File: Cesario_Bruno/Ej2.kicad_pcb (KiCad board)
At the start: 2 copper layers, 38.7 x 31.4 mm, 4 parts, among them P1 CONN_01X14, P2 CONN_01X14, X1 XTAL

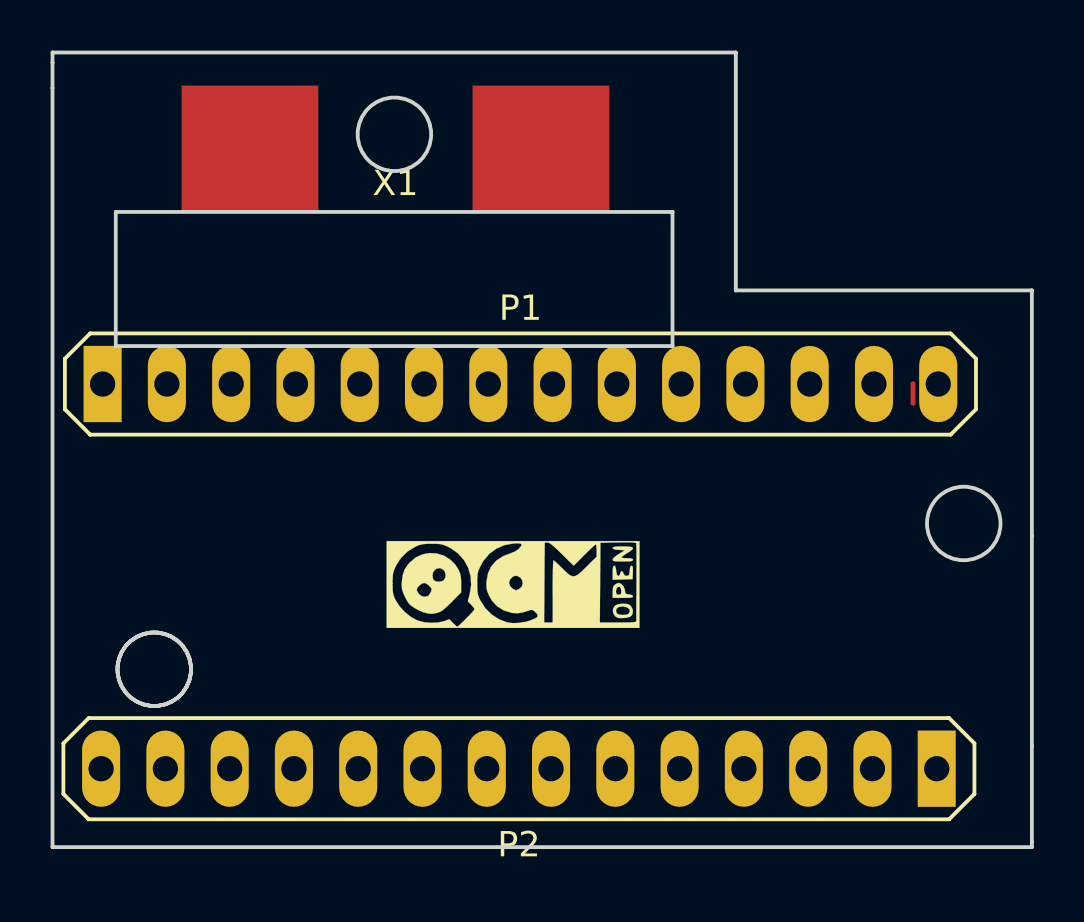
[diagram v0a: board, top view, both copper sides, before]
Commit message: Fin Clase 3. Generacion Nuevo PCB y Ruteo. Capa de Cobre. Archivos Gerber y Visualización.
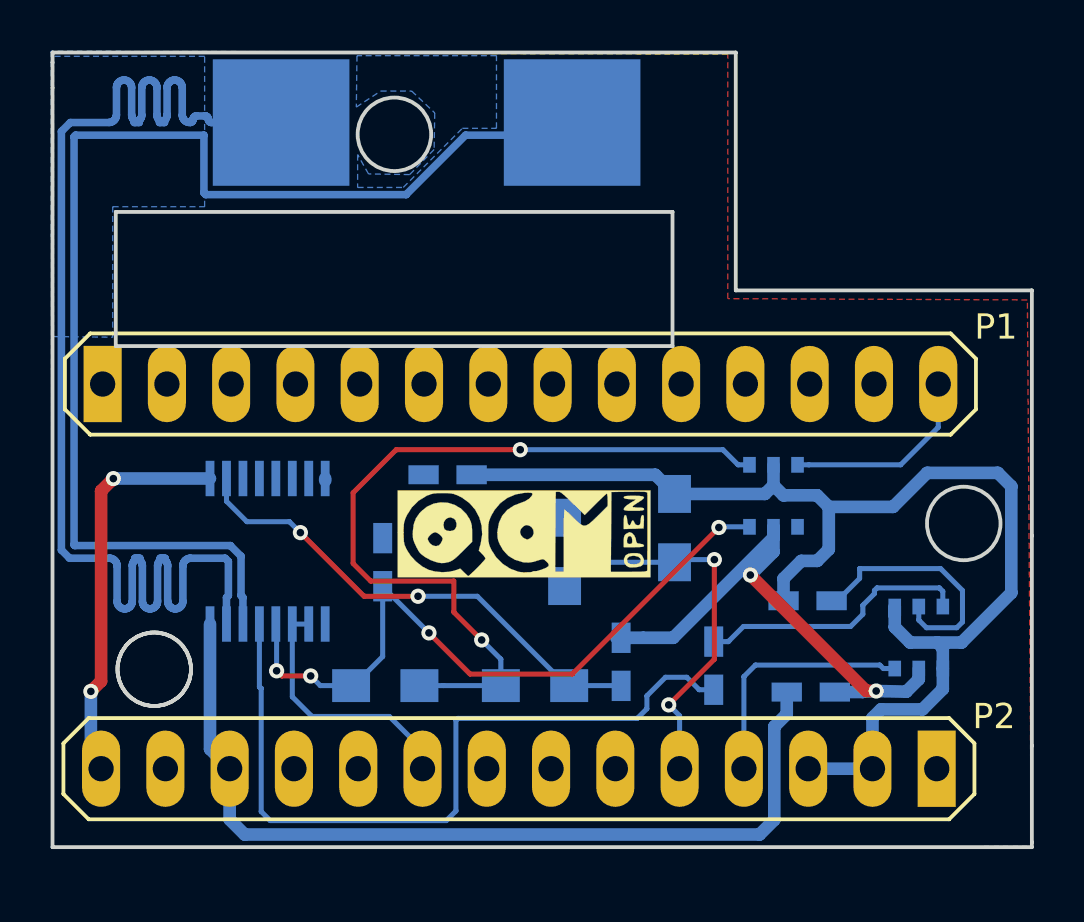
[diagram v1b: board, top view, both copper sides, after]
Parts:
- removed the G*** at (151.0, 105.0)
- added C1: 33pF, Ej2:C_0603_HandSoldering, B.Cu at (145.8, 104.1)
- added C2: 33pF, Ej2:C_0603_HandSoldering, B.Cu at (155.3, 108.1)
- added C3: 100nF, Ej2:C_0603_HandSoldering, B.Cu at (148.4, 100.7)
- added C4: pF, Ej2:C_0603_HandSoldering, B.Cu at (158.9, 108.2)
- added C5: pF, Ej2:C_0603_HandSoldering, B.Cu at (162.6, 105.7)
- added C6: 100nF, Ej2:C_0603_HandSoldering, B.Cu at (162.8, 109.3)
- added G***: LOGO, Ej2:openQCM, F.Cu at (151.4, 103.0)
- added PTC1: PTC_HandSoldering, Ej2:R_0805_HandSoldering, B.Cu at (153.0, 103.7)
- added R1: 1K, Ej2:R_0805_HandSoldering, B.Cu at (157.4, 102.8)
- added R2: 2M2, Ej2:R_0805_HandSoldering, B.Cu at (145.9, 109.0)
- added R3: 1K, Ej2:R_0805_HandSoldering, B.Cu at (151.9, 109.0)
- added U1: SN74LVC1GX04, Ej2:SOT-23-6, B.Cu at (162.2, 102.7)
- added U2: 74HCT4053, Ej2:TSSOP16, B.Cu at (141.3, 103.7)
- added U3: LTC5507, Ej2:SOT-23-6, B.Cu at (168.0, 108.3)
- P1, P2: footprint OpenQCM:PINHEAD1-14 -> Ej2:PINHEAD1-14
- X1: footprint OpenQCM:XTAL_con -> Ej2:XTAL_con; moved to B.Cu
- moved X1 2.16 mm to (147.6, 86.4)
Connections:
- P1 pad 1: (no net) -> Net-(P1-Pad1)
- P1 pad 10: (no net) -> Net-(P1-Pad10)
- P1 pad 11: (no net) -> Net-(P1-Pad11)
- P1 pad 12: (no net) -> Net-(P1-Pad12)
- P1 pad 13: (no net) -> Net-(P1-Pad13)
- P1 pad 14: /Arduino/FREQUENCY_IN -> /ArduinoCon/FREQUENCY_IN
- P1 pad 2: (no net) -> Net-(P1-Pad2)
- P1 pad 4: (no net) -> Net-(P1-Pad4)
- P1 pad 5: (no net) -> Net-(P1-Pad5)
- P1 pad 6: (no net) -> Net-(P1-Pad6)
- P1 pad 7: (no net) -> Net-(P1-Pad7)
- P1 pad 8: (no net) -> Net-(P1-Pad8)
- P1 pad 9: (no net) -> Net-(P1-Pad9)
- P2 pad 1: (no net) -> Net-(P2-Pad1)
- P2 pad 10: (no net) -> Net-(P2-Pad10)
- P2 pad 11: (no net) -> Net-(P2-Pad11)
- P2 pad 13: (no net) -> Net-(P2-Pad13)
- P2 pad 4: /Arduino/ENVELOPE_IN -> /ArduinoCon/ENVELOPE_IN
- P2 pad 5: /Arduino/PTC -> /ArduinoCon/PTC
- P2 pad 6: (no net) -> Net-(P2-Pad6)
- P2 pad 7: (no net) -> Net-(P2-Pad7)
- P2 pad 8: (no net) -> Net-(P2-Pad8)
- P2 pad 9: /Arduino/DIG_CONTROL -> /ArduinoCon/DIG_CONTROL
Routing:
- net /SWITCH_ENVELOPE/xtal_P: track 0.00 -> 55.6 mm
- net +3V3: track 0.00 -> 49.3 mm
- net /SWITCH_ENVELOPE/xtal_N: track 0.00 -> 48.8 mm
- net GND: track 0.00 -> 37.5 mm, vias 0 -> 4
- net +5V: track 0.00 -> 35.3 mm
- net Net-(R2-Pad1): track 0.00 -> 31.8 mm, vias 0 -> 2
- net Net-(C4-Pad1): track 0.00 -> 30.4 mm
- net /OSC_DRIVER/Switch_IN+: track 0.00 -> 27.9 mm, vias 0 -> 4
- net /OSC_DRIVER/Switch_IN-: track 0.00 -> 19.5 mm, vias 0 -> 2
- net /ArduinoCon/PTC: track 0.00 -> 15.9 mm, vias 0 -> 2
- net Net-(C4-Pad2): track 0.00 -> 10.9 mm
- net /ArduinoCon/DIG_CONTROL: track 0.00 -> 10.3 mm
- net Net-(C5-Pad2): track 0.00 -> 10.0 mm
- net /ArduinoCon/ENVELOPE_IN: track 0.00 -> 9.85 mm
- net /ArduinoCon/FREQUENCY_IN: track 0.00 -> 7.88 mm
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- added copper zone on B.Cu, net (none)
- added copper zone on B.Cu, net GND
- added copper zone on F.Cu, net GND
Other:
- net class Default: trace_width 0.2032 -> 0.2; via_drill 0.4 -> 0.3
- net class PW: via_drill 0.4 -> 0.3
- rule trace_min: 0.2032 -> 0.2
- rule via_min_size: 0.4 -> 0.6
